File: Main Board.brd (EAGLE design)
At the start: 82.5 x 38.1 mm, 25 parts, among them IC1 TB6612FNG, U1 TPS61030RSAR

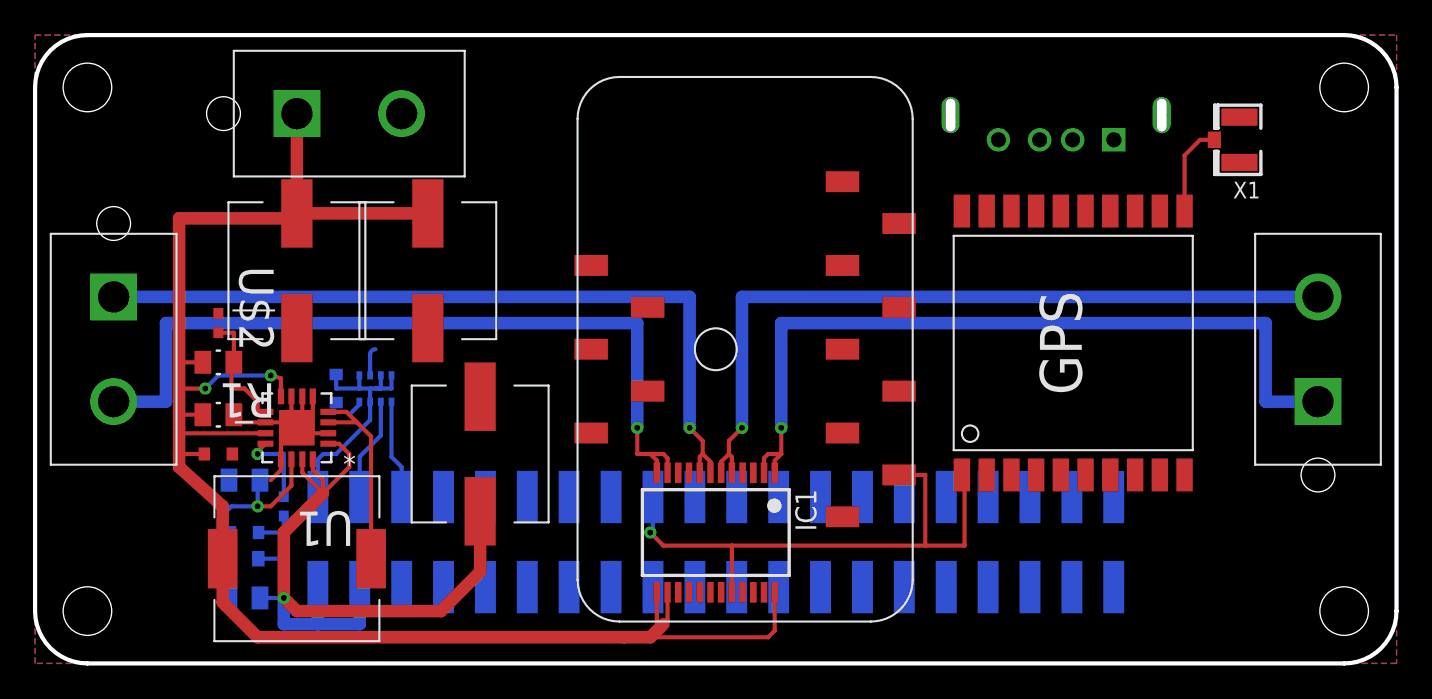
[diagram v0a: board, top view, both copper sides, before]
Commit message: Whatever man
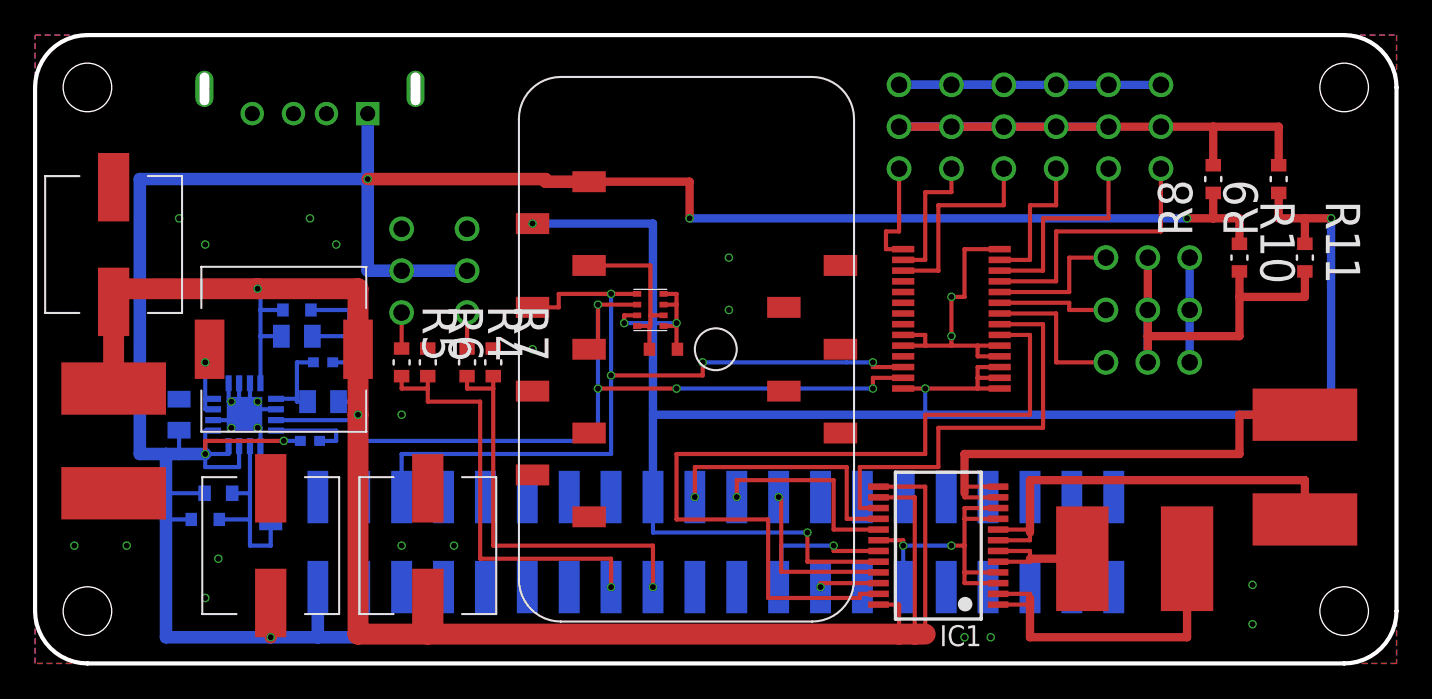
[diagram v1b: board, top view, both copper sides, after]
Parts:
- removed X1: (no value), Adafruit:U.FL
- added R10, R11, R4, R5, R6, R7, R8, R9: 1.65K Ohms, Vishay:RESC1608X60N
- added U$20, U$21: MOTOR, GoatFinder:MOTOR_PAD
- added U$22, U$23, U$24, U$25, U$26, U$28, U$29, U$30: PJUMP, GoatFinder:JUMPER
- added U$27: PWM, GoatFinder:TSSOP28
- U$15, U$16, U$17: value MOTOR2 -> PJUMP; device GoatFinder:BAT -> GoatFinder:JUMPER
- U$5: value GPS -> MOTOR; device GoatFinder:GPS -> GoatFinder:MOTOR_PAD
- moved U$15 55.8 mm to (-19.1, 4.76), turned to 180 degrees
- moved U$17 49.2 mm to (27.0, 13.5), turned to 180 degrees
- moved U$8 45.3 mm to (-24.6, 14.3)
- moved U$16 22.0 mm to (-15.1, 4.76), flipped to the bottom, turned to 180 degrees
- moved U$14 20.0 mm to (-3.17, 0.00), flipped to the top, turned to 0 degrees
- moved U$5 19.6 mm to (35.7, -7.14), turned to 0 degrees
- moved U$13 17.3 mm to (-3.97, 2.38), flipped to the top, turned to 180 degrees
- moved U$19 16.7 mm to (-17.5, -11.9), turned to 270 degrees
- moved U$12 13.9 mm to (-27.0, -11.9)
- moved IC1 13.5 mm to (13.5, -11.9), turned to 90 degrees
- moved U$1 12.7 mm to (-26.2, 0.00), turned to 0 degrees
- moved U$9 11.8 mm to (-32.5, -3.97), turned to 90 degrees
- moved U$18 11.2 mm to (-36.5, 6.35), turned to 270 degrees
- moved U$7 9.95 mm to (-25.4, 2.38), flipped to the bottom, turned to 0 degrees
- moved R1 6.78 mm to (-23.8, -3.17), flipped to the bottom
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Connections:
- removed net GPIO4: U$11.GPIO4, U$5.P$5
- removed net GPIO5: U$11.GPIO5, U$5.P$2
- removed net N$13: U$11.SDA0, U$6.P$24
- removed net N$14: U$11.SCL0, U$6.P$23
- removed net N$4: U$11.TXD, U$5.P$10
- removed net PWMA: U$11.GPIO23
- removed net PWMB: U$11.GPIO26
- new net HALL1: R5.2, R6.2, U$11.GPIO4
- new net HALL2: R4.2, R7.2, U$11.GPIO5
- new net N$5: R5.1, U$15.VIN@1
- new net N$6: R4.1, U$16.VIN@1
- new net PWM0: U$27.P$8, U$30.VIN@1
- new net PWM1: U$27.P$9, U$29.VIN@1
- new net PWM10: U$26.VIN@1, U$27.P$17
- new net PWM2: U$27.P$10, U$28.VIN@1
- new net PWM5: U$17.VIN@1, U$27.P$11
- new net PWM6: U$22.VIN@1, U$27.P$12
- new net PWM7: U$23.VIN@1, U$27.P$13
- new net PWM8: U$24.VIN@1, U$27.P$15
- new net PWM9: U$25.VIN@1, U$27.P$16
- net +3.3V: now also R11.1, R9.1, U$27.P$1, U$27.P$2, U$27.P$28, U$27.P$3; no longer U$5.P$1
- net +5V: now also R10.1, R8.1, U$15.VIN@2, U$16.VIN@2
- net GND: now also R6.1, R7.1, U$15.VOUT, U$16.VOUT, U$17.VOUT, U$21.P$2, U$22.VOUT, U$23.VOUT, U$24.VOUT, U$25.VOUT, U$26.VOUT, U$27.P$14, U$27.P$23, U$27.P$24, U$27.P$4, U$27.P$5, U$28.VOUT, U$29.VOUT, U$30.VOUT; no longer U$17.P$2, U$5.P$12, U$5.P$19, U$5.P$3, U$5.P$8, X1.1, X1.2
- net GPIO0: no longer U$5.P$13
- net MOTA: now also U$27.P$6
- net MOTB: now also U$27.P$7
- net N$10: now also U$27.P$26, U$6.P$23
- net N$12: now also U$27.P$27, U$6.P$24
- net N$16: now also U$20.P$1; no longer U$15.P$1
- net N$17: now also U$20.P$2; no longer U$15.P$2
- net N$18: now also U$5.P$1; no longer U$16.P$1
- net N$19: now also U$5.P$2; no longer U$16.P$2
- net N$3: now also R8.2, R9.2, U$17.VIN@2, U$22.VIN@2, U$23.VIN@2, U$24.VIN@2, U$25.VIN@2, U$26.VIN@2; no longer U$11.RXD, U$5.P$9
- net N$8: now also R10.2, R11.2, U$28.VIN@2, U$29.VIN@2, U$30.VIN@2; no longer U$5.P$11, X1.3
- net VBAT: now also U$21.P$1; no longer U$17.P$1
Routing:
- net +5V: track 53.9 -> 159.1 mm, vias 1 -> 6
- net +3.3V: track 50.0 -> 150.8 mm, vias 1 -> 6
- net GND: track 19.7 -> 105.7 mm, vias 0 -> 26
- net MOTA: track 0.00 -> 51.7 mm
- net N$3: track 0.00 -> 46.7 mm
- net N$10: track 6.03 -> 51.1 mm, vias 0 -> 4
- net N$12: track 6.31 -> 50.9 mm, vias 0 -> 4
- net N$17: track 47.3 -> 7.69 mm, vias 1 -> 0
- net N$16: track 48.6 -> 21.2 mm, vias 1 -> 0
- net HALL1: track 0.00 -> 26.2 mm, vias 0 -> 1
- net MOTB: track 0.00 -> 26.0 mm
- net HALL2: track 0.00 -> 24.8 mm, vias 0 -> 1
- net N$18: track 47.3 -> 26.7 mm, vias 1 -> 0
- net N$8: track 5.57 -> 24.5 mm
- net N$19: track 48.6 -> 30.1 mm, vias 1 -> 0
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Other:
- board text added: "+"
- board text added: "-"
- board text added: "0"
- board text added: "1"
- board text added: "10"
- board text added: "2"
- board text added: "3"
- board text added: "3V"
- board text added: "4"
- board text added: "5"
- board text added: "5V"
- board text added: "6"
- board text added: "7"
- board text added: "8"
- board text added: "9"
- board text added: "GND"
- board text added: "GoatFinder V1"
- board text added: "Vin"
